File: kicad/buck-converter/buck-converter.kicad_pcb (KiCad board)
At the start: 2 copper layers, 51 parts, among them J1 Screw_Terminal_01x02, J2 Screw_Terminal_01x02, Q1 IRLZ44N, Q10 2N2222, Q11 2N2222, Q12 2N2907, Q7 2N2222, Q8 BC327-25, Q9 2N2222, U1 TL431LP, U3 NE555, U6 LM358, U7 LM393

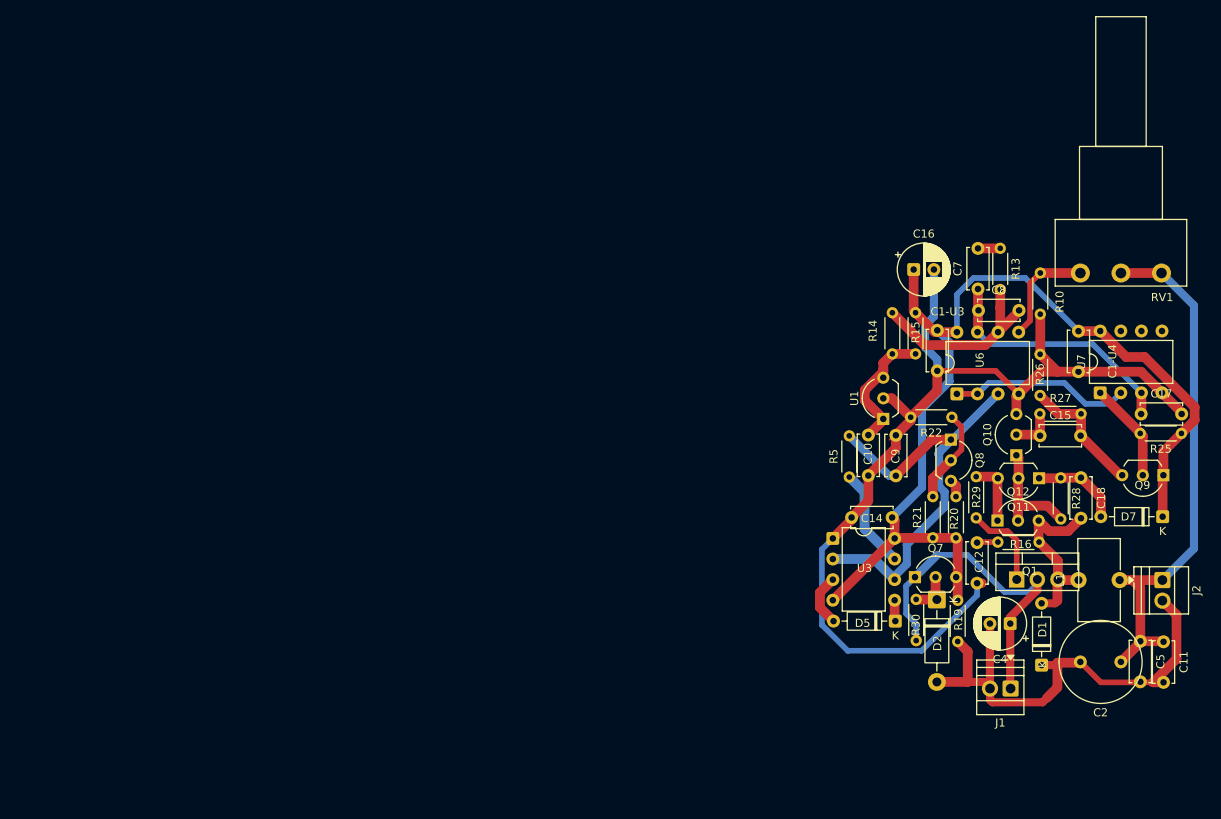
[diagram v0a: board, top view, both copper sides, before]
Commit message: Finalized perfboard PCB design.
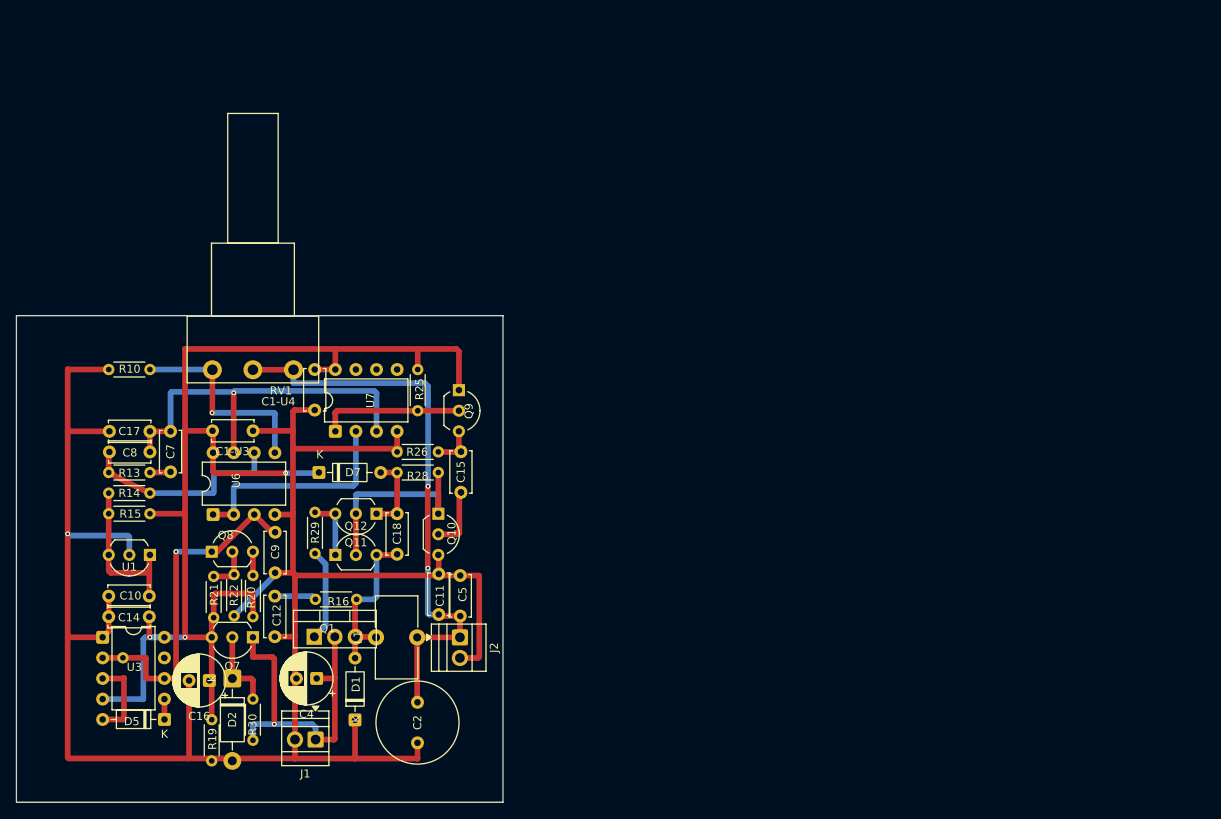
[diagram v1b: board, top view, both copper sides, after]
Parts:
- R27, R5: moved to B.Cu
- moved C17 122.2 mm to (64.3, 99.1), turned to 180 degrees
- moved R10 110.4 mm to (64.3, 91.4), turned to 180 degrees
- moved R13 108.4 mm to (64.3, 104.1), turned to 180 degrees
- moved RV1 107.7 mm to (82.0, 91.5)
- moved D7 104.2 mm to (85.1, 104.1), turned to 0 degrees
- moved C8 103.7 mm to (64.3, 101.6), turned to 180 degrees
- moved C7 101.1 mm to (66.8, 99.1), turned to -90 degrees
- moved C16 100.6 mm to (71.6, 129.8), turned to 180 degrees
- moved R15 97.6 mm to (64.3, 109.2), turned to 180 degrees
- moved R25 94.5 mm to (97.3, 91.4), turned to -90 degrees
- moved U7 94.4 mm to (87.1, 99.1)
- moved C1-U4 94.3 mm to (84.6, 91.4)
- moved R14 94.2 mm to (64.3, 106.7), turned to 180 degrees
- moved R19 93.2 mm to (71.9, 134.6)
- moved U6 92.9 mm to (72.0, 109.3)
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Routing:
- net GND: track 189.9 -> 255.6 mm, vias 0 -> 1
- net REGULATED_VCC: track 123.6 -> 156.7 mm, vias 0 -> 3
- net DUTY_CTRL_VOLTAGE: track 31.3 -> 47.5 mm, vias 0 -> 1
- net SAWTOOTH: track 56.3 -> 42.3 mm, vias 0 -> 1
- net Net-(U3-DIS): track 12.4 -> 0.04 mm
- net FB: track 13.3 -> 25.6 mm, vias 0 -> 1
- net Net-(Q10-C): track 14.1 -> 25.0 mm
- net Net-(Q9-E): track 15.9 -> 5.25 mm
- net Net-(Q8-B): track 11.7 -> 5.52 mm
- net SWITCH: track 12.3 -> 17.7 mm
- net Net-(U6A--): track 22.4 -> 27.6 mm
- net CONVERTER_OUTPUT: track 66.4 -> 71.5 mm, vias 0 -> 2
- net Net-(D2-K): track 5.39 -> 10.0 mm
- net Net-(D5--): track 6.48 -> 10.3 mm
- net Net-(U1-K): track 17.0 -> 19.8 mm
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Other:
- board outline added: 60 x 60 mm
